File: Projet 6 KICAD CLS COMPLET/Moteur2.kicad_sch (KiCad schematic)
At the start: 11 parts, among them SW1 SW_DIP_x02

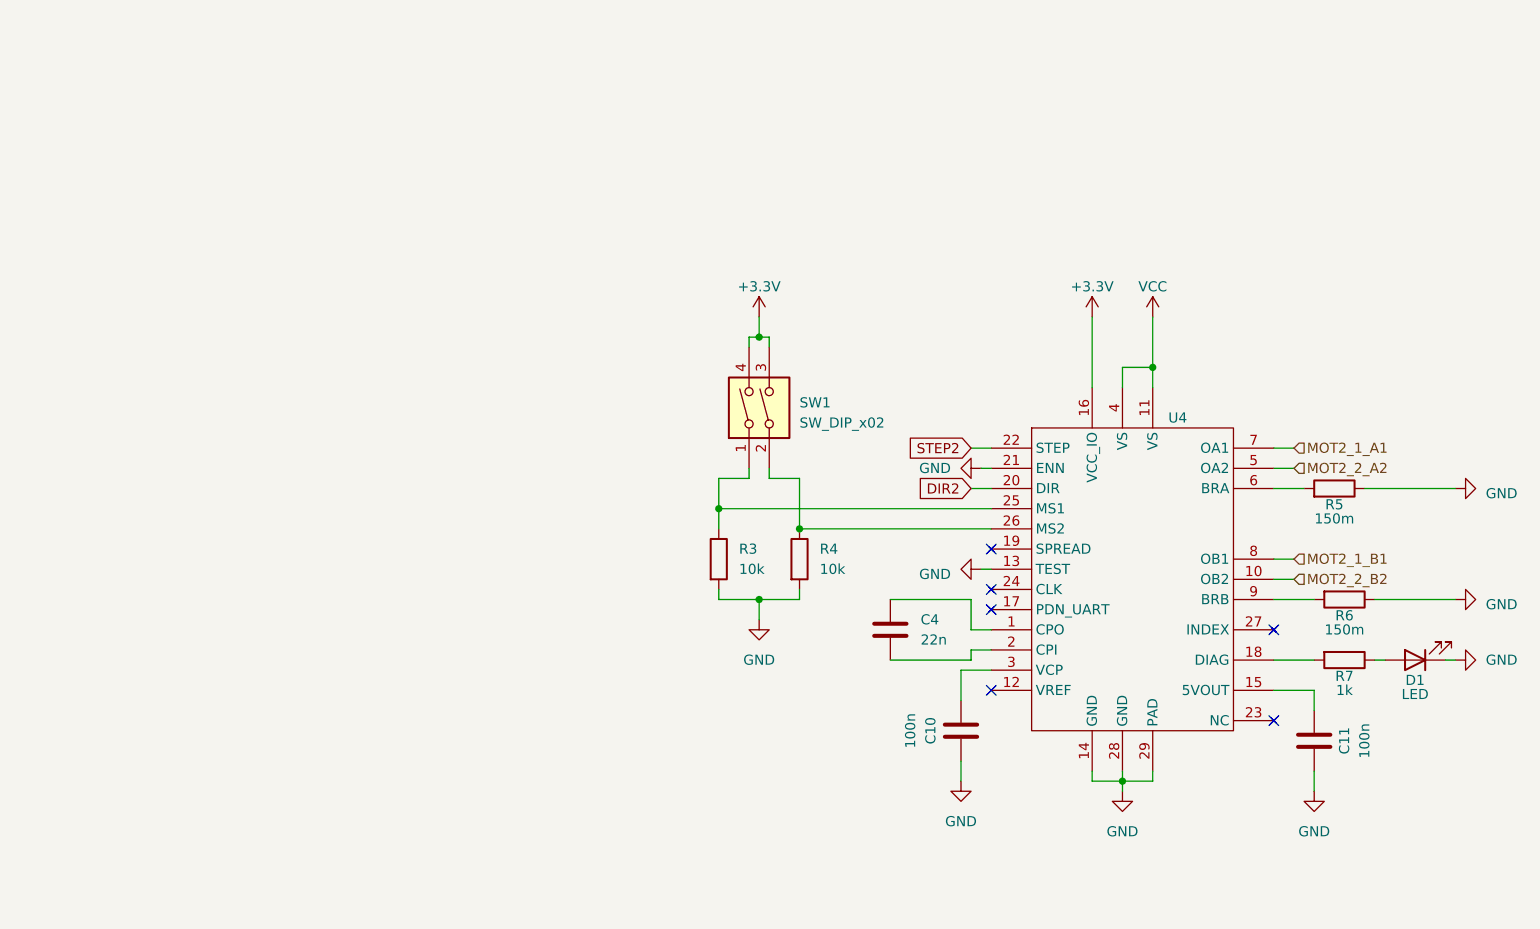
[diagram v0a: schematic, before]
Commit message: Projet 6 KICAD CLS COMPLET Correction
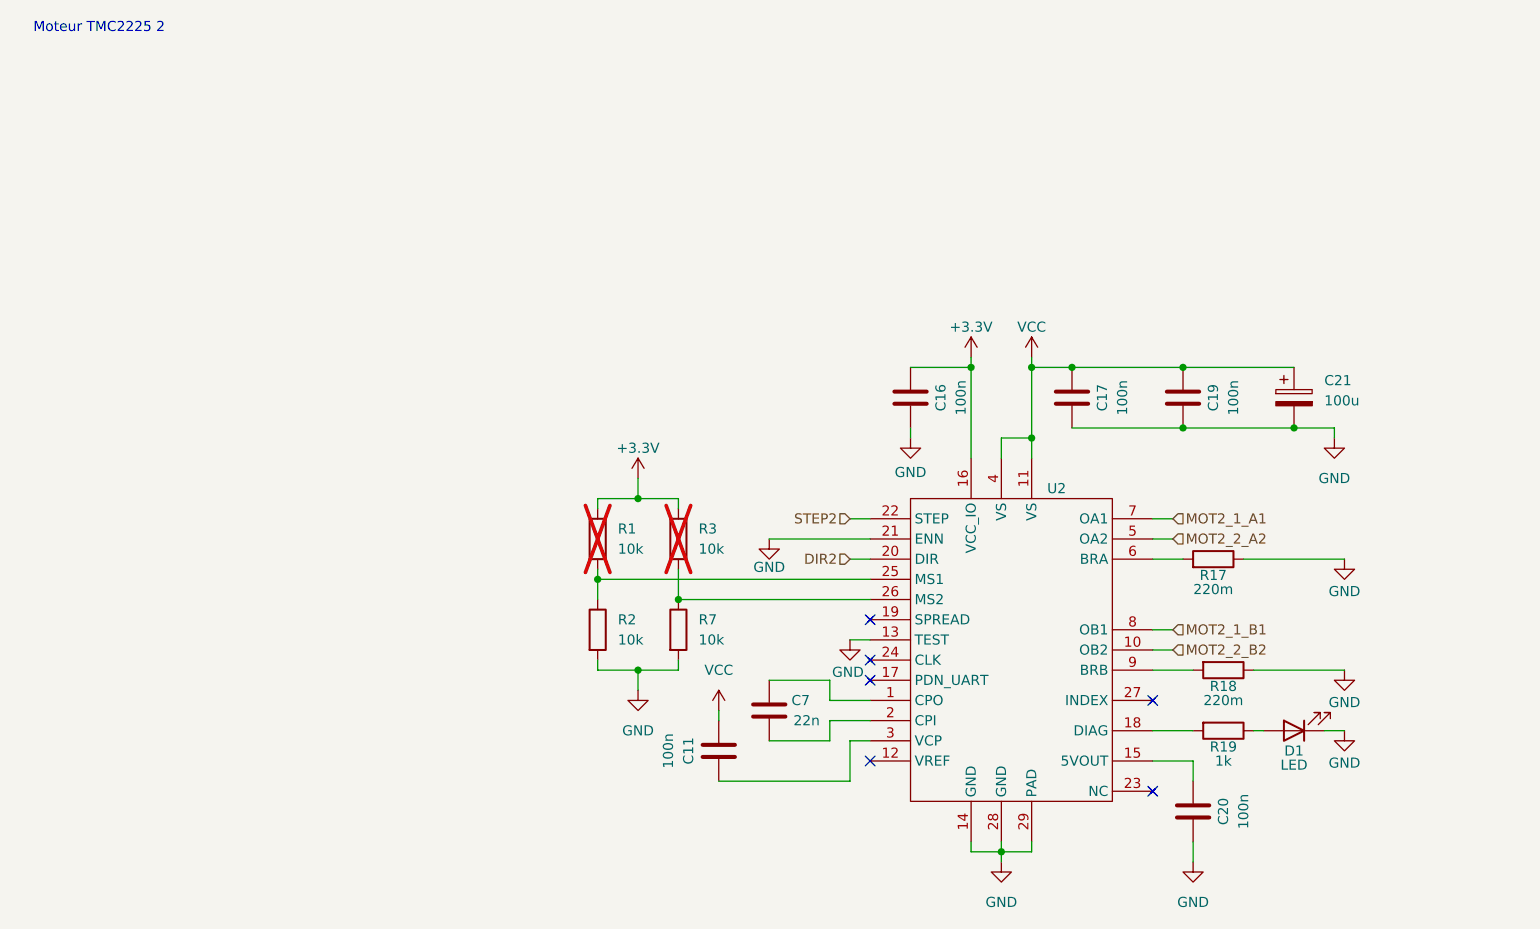
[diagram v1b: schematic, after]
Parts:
- removed C10: 100n, symbol Device:C
- removed C4: 22n, symbol Device:C
- removed R4: 10k, symbol Device:R
- removed R5, R6: 150m, symbol Device:R
- removed SW1: SW_DIP_x02, symbol Switch:SW_DIP_x02
- removed U4: ~, symbol My_Lib:TMC2225
- added C16, C17, C19, C20: 100n, symbol Device:C
- added C21: 100u, symbol Device:C_Polarized
- added C7: 22n, symbol Device:C
- added R1, R2: 10k, symbol Device:R
- added R17, R18: 220m, symbol Device:R
- added R19: 1k, symbol Device:R
- added U2: ~, symbol My_Lib:TMC2225
- R3: now not fitted
- R7: value 1k -> 10k
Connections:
- net +3.3V: now also R3.1, C16.1, R1.1, U2.16 (VCC_IO)
- net DIR2: now also U2.20 (DIR)
- net GND: now also R7.2, C16.2, C17.2, C19.2, C20.2, C21.2, R17.1, R18.1, R2.2, U2.13 (TEST), U2.14 (GND), U2.21 (ENN), U2.28 (GND), U2.29 (PAD); no longer C11.2, R3.2
- net MOT2_1_A1: now also U2.7 (OA1)
- net MOT2_1_B1: now also U2.8 (OB1)
- net MOT2_2_A2: now also U2.5 (OA2)
- net MOT2_2_B2: now also U2.10 (OB2)
- net STEP2: now also U2.22 (STEP)
- net VCC: now also C11.2, C17.1, C19.1, C21.1, U2.11 (VS), U2.4 (VS)
- net at R7.1: now also R3.2, U2.26 (MS2); no longer D1.2 (A)
- net at C11.1: now also U2.3 (VCP)
- new net: C7.1, U2.1 (CPO)
- new net: C20.1, U2.15 (5VOUT)
- new net: R19.2, U2.18 (DIAG)
- new net: C7.2, U2.2 (CPI)
- new net: R1.2, R2.1, U2.25 (MS1)
- new net: R17.2, U2.6 (BRA)
- new net: R18.2, U2.9 (BRB)
- new net: D1.2 (A), R19.1
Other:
- note added: "Moteur TMC2225 2"
